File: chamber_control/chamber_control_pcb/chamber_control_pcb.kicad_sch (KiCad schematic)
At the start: 27 parts, among them Q1 2N2222, Q2 2N2222, SW1 GAS_IN, SW2 GAS_OUT

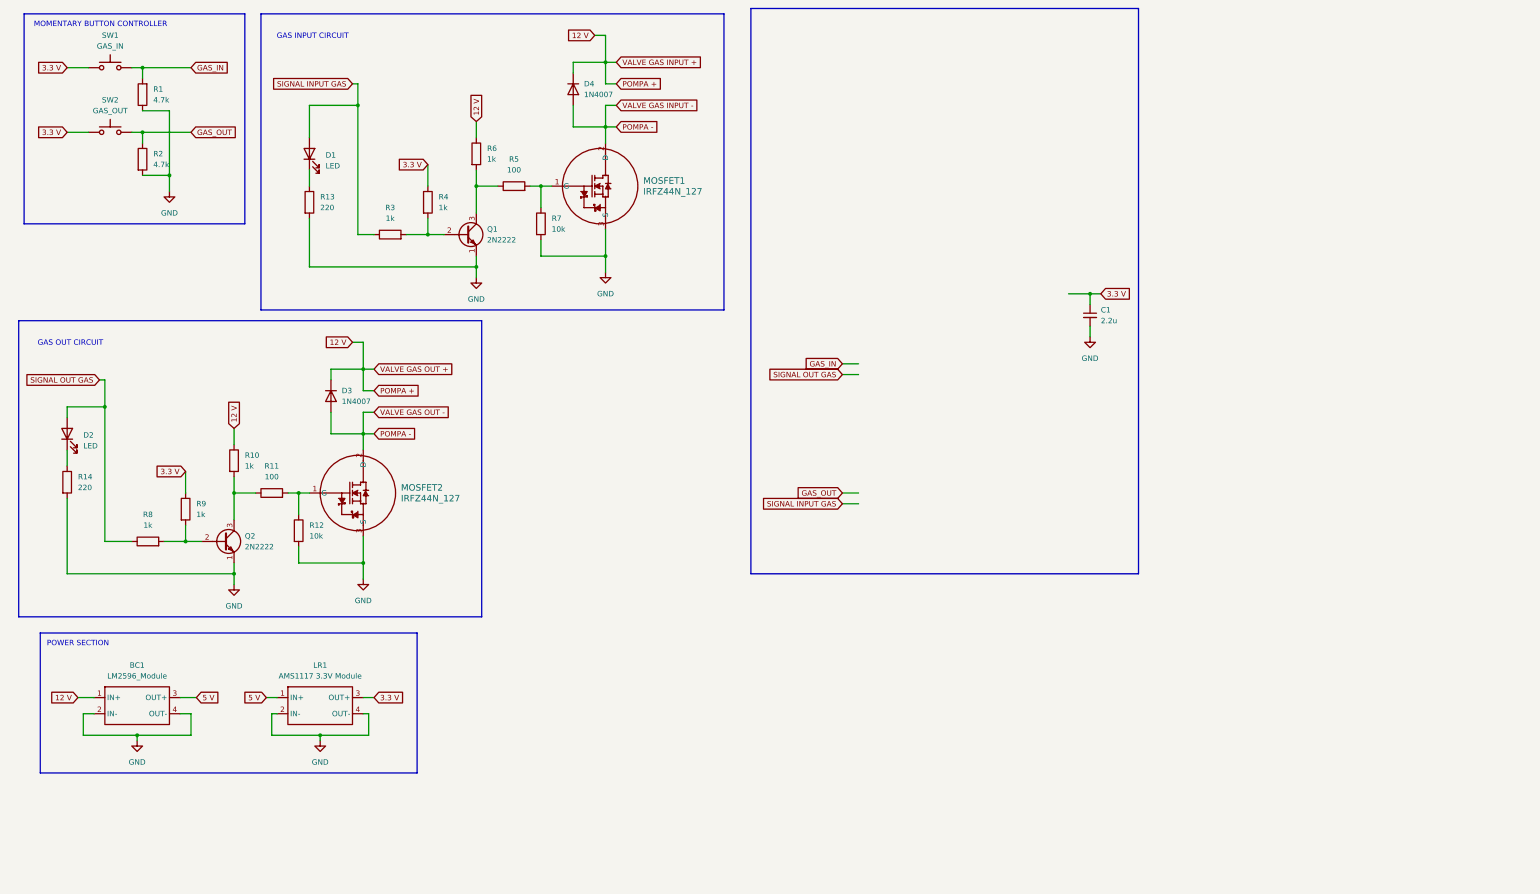
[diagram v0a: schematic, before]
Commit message: update control chamber pcb
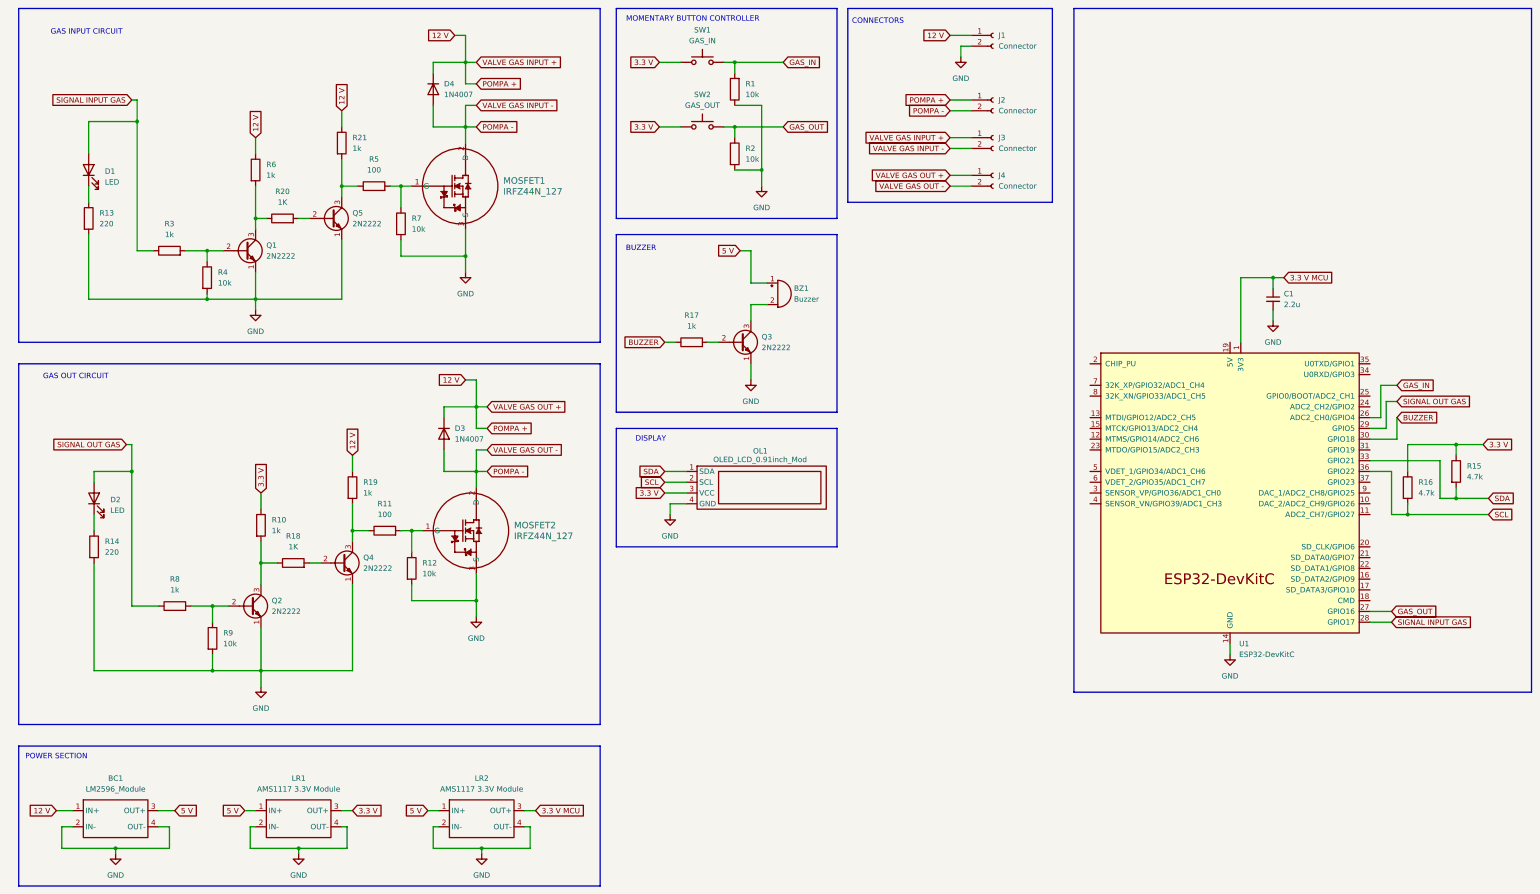
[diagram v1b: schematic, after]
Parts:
- added BZ1: Buzzer, symbol Device:Buzzer
- added J1, J2, J3, J4: Connector, symbol Connector:Conn_01x02_Socket
- added LR2: AMS1117 3.3V Module, symbol Linear_Voltage_Regulator_Module:AMS1117_3V3_Module
- added OL1: OLED_LCD_0.91inch_Mod, symbol OLED_LCD_Module:OLED_LCD_0.91_inch_Module
- added Q3, Q4, Q5: 2N2222, Package_TO_SOT_THT:TO-39-3, symbol Transistor_BJT:2N2219
- added R15, R16: 4.7k, symbol Device:R
- added R17, R19, R21: 1k, symbol Device:R
- added R18, R20: 1K, symbol Device:R
- added U1: ESP32-DevKitC, Espressif:ESP32-DevKitC, symbol Espressif:ESP32-DevKitC
- R1, R2: value 4.7k -> 10k
- R4, R9: value 1k -> 10k
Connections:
- net 12 V: now also J1.1 (Pin_1), J2.1 (Pin_1), J3.1 (Pin_1), J4.1 (Pin_1), R19.1, R21.1; no longer R10.1
- net 3.3 V: now also R10.1, OL1.3 (VCC), R15.1, R16.1; no longer C1.1, R4.1, R9.1
- net 5 V: now also BZ1.1 (+), LR2.1 (IN+)
- net GAS_IN: now also U1.26 (ADC2_CH0/GPIO4)
- net GAS_OUT: now also U1.27 (GPIO16)
- net GND: now also R4.2, R9.2, J1.2 (Pin_2), LR2.2 (IN-), LR2.4 (OUT-), OL1.4 (GND), Q3.1 (E), Q4.1 (E), Q5.1 (E), U1.14 (GND), U1.32 (GND), U1.38 (GND)
- net POMPA -: now also J2.2 (Pin_2), J3.2 (Pin_2), J4.2 (Pin_2)
- net SIGNAL INPUT GAS: now also U1.28 (GPIO17)
- net SIGNAL OUT GAS: now also U1.29 (GPIO5)
- net at Q1.3 (C), R6.2: now also R20.1; no longer R5.1
- net at Q1.2 (B), R3.2: now also R4.1; no longer R4.2
- net at Q2.2 (B), R8.2: now also R9.1; no longer R9.2
- net at Q2.3 (C), R10.2: now also R18.1; no longer R11.1
- new net: Q5.3 (C), R21.2, R5.1
- new net: Q4.3 (C), R11.1, R19.2
- new net: Q5.2 (B), R20.2
- new net: Q4.2 (B), R18.2
- new net: Q3.2 (B), R17.2
- new net: BZ1.2 (-), Q3.3 (C)
- new net 3.3 V MCU: C1.1, LR2.3 (OUT+), U1.1 (3V3)
- new net BUZZER: R17.1, U1.30 (GPIO18)
- new net SCL: OL1.2 (SCL), R16.2, U1.36 (GPIO22)
- new net SDA: OL1.1 (SDA), R15.2, U1.33 (GPIO21)
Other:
- note added: "BUZZER"
- note added: "CONNECTORS"
- note added: "DISPLAY"
- moved on the sheet: BC1, C1, D1, D2, D3, D4, LR1, MOSFET1, MOSFET2, Q1, Q2, R1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
